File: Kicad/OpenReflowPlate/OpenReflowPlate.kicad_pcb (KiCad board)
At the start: 2 copper layers, 7 parts, among them U1 STM32L476RGTx

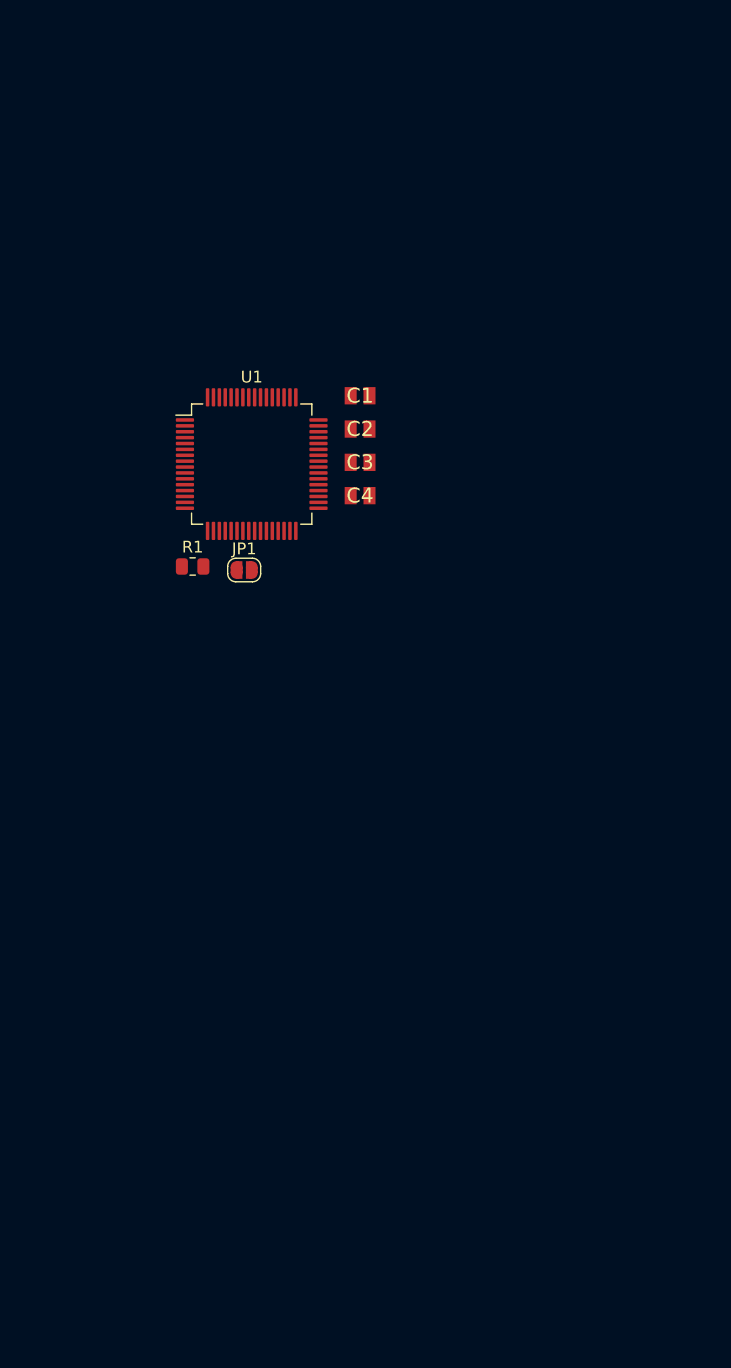
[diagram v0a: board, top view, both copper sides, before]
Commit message: last version
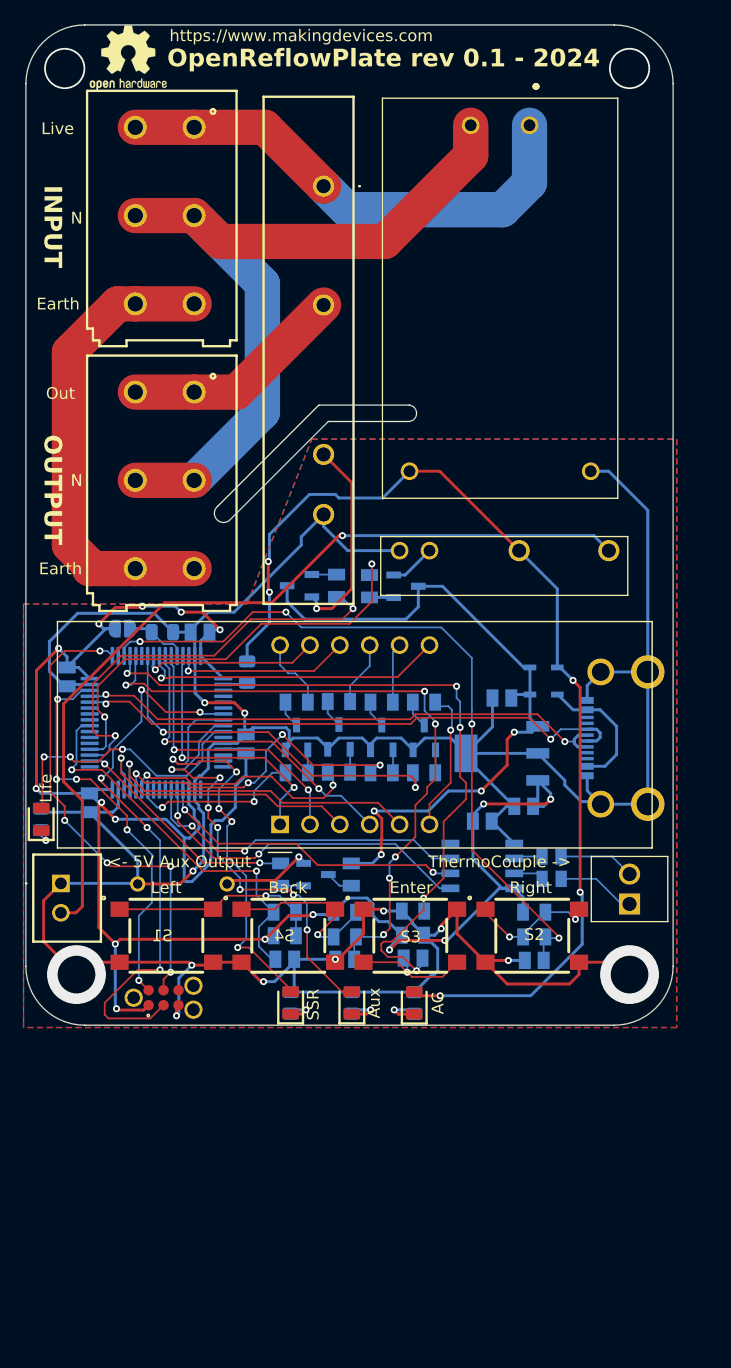
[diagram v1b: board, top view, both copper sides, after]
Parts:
- added AC/DC 3w: HLK-PM03, User_lib:HLKPM03, F.Cu at (129.5, 25.8)
- added Buzzer: TMB12A05, User_lib:TMB12A05, B.Cu at (103.8, 90.3)
- added C1: 100nF, User_lib:CAPC2012X140N, B.Cu at (125.5, 85.0)
- added C10: 22pF, User_lib:CAPC2012X140N, B.Cu at (113.8, 96.7)
- added C11: 22pF, User_lib:CAPC2012X140N, B.Cu at (119.6, 96.6)
- added C2: 100nF, User_lib:CAPC2012X140N, B.Cu at (127.2, 74.5)
- added C3: 100nF, User_lib:CAPC2012X140N, B.Cu at (129.0, 83.7)
- added C8: 22pF, User_lib:CAPC2012X140N, B.Cu at (129.9, 96.8)
- added C9: 22pF, User_lib:CAPC2012X140N, B.Cu at (108.7, 96.7)
- added D1: ZLLS410TA, User_lib:SOD2513X120N, B.Cu at (130.7, 74.2)
- added D2: ZLLS410TA, User_lib:SOD2513X120N, B.Cu at (130.7, 71.9)
- added IC1: MAX31855KASA+, User_lib:SOIC127P600X175-8N, B.Cu at (125.5, 88.8)
- added IC2: TC1108-3.3VDBTR, User_lib:SOT230P700X180-4N, B.Cu at (127.2, 79.2)
- added J1: TC connector, User_lib:282834-2_1, F.Cu at (138.0, 92.0)
- added J2: B2B-XH-A, User_lib:B2BXHA, F.Cu at (89.7, 90.2)
- added J3: Output_AC, User_lib:691411910003, F.Cu at (98.5, 56.0)
- added J4: Input_AC, User_lib:691411910003, F.Cu at (98.5, 33.5)
- added J5: Type - C, User_lib:2169900003, B.Cu at (138.4, 77.9)
- added K1: SSRC-240D5R, User_lib:SSRC240D5R, F.Cu at (112.0, 31.0)
- added K2: HF49FD_012-1H12F, User_lib:HF49FD0121H12F, F.Cu at (136.2, 62.0)
- added LED1: SML-H12V8TT86, User_lib:LEDC2012X90N, F.Cu at (119.7, 100.4)
- added LED2: SML-H12V8TT86, User_lib:LEDC2012X90N, F.Cu at (109.2, 100.4)
- added LED3: SML-H12V8TT86, User_lib:LEDC2012X90N, F.Cu at (114.4, 100.4)
- added LED4: SML-H12V8TT86, User_lib:LEDC2012X90N, F.Cu at (88.0, 84.8)
- added LFB1: Ferrite, User_lib:CAPC2012X90N, B.Cu at (131.4, 88.0)
- added LFB2: Ferrite, User_lib:CAPC2012X90N, B.Cu at (131.4, 89.9)
- added Q1: SMMBT5551LT1G, User_lib:SOT96P237X111-3N, B.Cu at (109.7, 77.8)
- added Q2: SMMBT5551LT1G, User_lib:SOT96P237X111-3N, B.Cu at (113.3, 77.8)
- added Q3: SMMBT5551LT1G, User_lib:SOT96P237X111-3N, B.Cu at (116.9, 77.8)
- added Q4: SMMBT5551LT1G, User_lib:SOT96P237X111-3N, B.Cu at (120.6, 77.8)
- added Q5: SMMBT5551LT1G, User_lib:SOT96P237X111-3N, B.Cu at (111.3, 89.5)
- added Q6: SMMBT5551LT1G, User_lib:SOT96P237X111-3N, B.Cu at (110.0, 65.0)
- added Q7: SMMBT5551LT1G, User_lib:SOT96P237X111-3N, B.Cu at (119.0, 65.0)
- added R1: 4k7, User_lib:RESC2012X65N, B.Cu at (109.7, 80.8)
- added R10: 100, User_lib:RESC2012X65N, B.Cu at (116.9, 74.8)
- added R11: 4k7, User_lib:RESC2012X65N, B.Cu at (120.5, 80.8)
- added R12: 100, User_lib:RESC2012X65N, B.Cu at (120.5, 74.8)
- added R13: 0, Resistor_SMD:R_0805_2012Metric, B.Cu at (105.5, 72.3)
- added R15: 10k, User_lib:RESC2012X75N, B.Cu at (129.9, 94.8)
- added R16: 10k, User_lib:RESC2012X75N, B.Cu at (108.7, 94.7)
- added R17: 10K, User_lib:RESC2012X65N, B.Cu at (108.7, 92.7)
- added R18: 10k, User_lib:RESC2012X65N, B.Cu at (129.9, 92.7)
- added R19: 4k7, User_lib:RESC2012X65N, B.Cu at (108.3, 89.5)
- added R2: 1k, Resistor_SMD:R_0805_2012Metric, B.Cu at (119.7, 100.4)
- added R20: 220, User_lib:RESC2012X65N, B.Cu at (114.3, 89.5)
- added R21: 10K, User_lib:RESC2012X75N, B.Cu at (119.6, 92.6)
- added R22: 10k, User_lib:RESC2012X75N, B.Cu at (113.8, 94.8)
- added R23: 4k7, User_lib:RESC2012X65N, B.Cu at (113.1, 65.0)
- added R24: 10k, User_lib:RESC2012X65N, B.Cu at (119.6, 94.7)
- added R25: 10k, User_lib:RESC2012X65N, B.Cu at (113.8, 92.7)
- added R26: 4k7, User_lib:RESC2012X65N, B.Cu at (115.9, 65.0)
- added R3: 100, User_lib:RESC2012X65N, B.Cu at (109.7, 74.8)
- added R4: 220, Resistor_SMD:R_0805_2012Metric, B.Cu at (109.2, 100.4)
- added R5: 4k7, User_lib:RESC2012X65N, B.Cu at (113.3, 80.8)
- added R6: 100, User_lib:RESC2012X65N, B.Cu at (113.3, 74.8)
- added R7: 220, Resistor_SMD:R_0805_2012Metric, B.Cu at (114.4, 100.4)
- added R8: 220, Resistor_SMD:R_0805_2012Metric, B.Cu at (88.0, 84.8)
- added R9: 4k7, User_lib:RESC2012X65N, B.Cu at (116.9, 80.8)
- added REF**: OSHW-Logo2_7.3x6mm_SilkScreen, Symbol:OSHW-Logo2_7.3x6mm_SilkScreen, F.Cu at (95.4, 20.1)
- added S1: Left Button, User_lib:430182070816, F.Cu at (98.6, 94.7)
- added S2: Right Button, User_lib:430182070816, F.Cu at (129.7, 94.7)
- added S3: Enter Button, User_lib:430182070816, F.Cu at (119.4, 94.7)
- added S4: Back Button, User_lib:430182070816, F.Cu at (109.0, 94.7)
- added SWD: TC2030-MCP-NL, User_lib:TC2030-MCP-NL, F.Cu at (98.4, 100.0)
- added U1: CC56-12EWA, Display_7Segment:CA56-12EWA, F.Cu at (108.3, 85.2)
- C4: renamed from C1; moved to B.Cu
- C5: renamed from C2; moved to B.Cu
- C6: renamed from C3; moved to B.Cu
- C7: renamed from C4; moved to B.Cu
- JP1: moved to B.Cu
- R14: renamed from R1; moved to B.Cu
- U2: renamed from U1; moved to B.Cu
- moved C7 34.8 mm to (92.1, 83.4), turned to 90 degrees
- moved C5 32.6 mm to (90.2, 72.7), turned to 90 degrees
- moved C4 31.1 mm to (105.4, 78.4), turned to -90 degrees
- moved U2 23.4 mm to (97.8, 76.6), turned to 180 degrees
- moved C6 19.8 mm to (101.5, 68.9)
- moved JP1 11.5 mm to (94.9, 68.6)
- moved R14 6.14 mm to (98.3, 68.9), turned to 180 degrees
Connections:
- U2 pad 10: unconnected-(U1-PC2-Pad10) -> LED_LIFE
- U2 pad 2: unconnected-(U1-PC13-Pad2) -> Net-(U2-PC13)
- U2 pad 20: unconnected-(U1-PA4-Pad20) -> SPI1_NSS
- U2 pad 21: unconnected-(U1-PA5-Pad21) -> SPI_CLK
- U2 pad 22: unconnected-(U1-PA6-Pad22) -> SPI_MISO
- U2 pad 26: unconnected-(U1-PB0-Pad26) -> C_1
- U2 pad 27: unconnected-(U1-PB1-Pad27) -> C_2
- U2 pad 28: unconnected-(U1-PB2-Pad28) -> C_3
- U2 pad 29: unconnected-(U1-PB10-Pad29) -> D_g
- U2 pad 30: unconnected-(U1-PB11-Pad30) -> D_dp
- U2 pad 34: unconnected-(U1-PB13-Pad34) -> C_buzzer
- U2 pad 35: unconnected-(U1-PB14-Pad35) -> C_out1
- U2 pad 36: unconnected-(U1-PB15-Pad36) -> C_out2
- U2 pad 40: unconnected-(U1-PC9-Pad40) -> BUT_LEFT
- U2 pad 51: unconnected-(U1-PC10-Pad51) -> BUT_RIGHT
- U2 pad 52: unconnected-(U1-PC11-Pad52) -> BUT_ENTER
- U2 pad 53: unconnected-(U1-PC12-Pad53) -> BUT_BACK
- U2 pad 55: unconnected-(U1-PB3-Pad55) -> C_4
- U2 pad 56: unconnected-(U1-PB4-Pad56) -> D_a
- U2 pad 57: unconnected-(U1-PB5-Pad57) -> D_b
- U2 pad 58: unconnected-(U1-PB6-Pad58) -> D_c
- U2 pad 59: unconnected-(U1-PB7-Pad59) -> D_d
- U2 pad 61: unconnected-(U1-PB8-Pad61) -> D_e
- U2 pad 62: unconnected-(U1-PB9-Pad62) -> D_f
- U2 pad 7: unconnected-(U1-NRST-Pad7) -> reset
- U2 pad 8: unconnected-(U1-PC0-Pad8) -> LED_OUT1
- U2 pad 9: unconnected-(U1-PC1-Pad9) -> LED_OUT2
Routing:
- net GND: track 0.00 -> 299.6 mm, vias 0 -> 12
- net +3V3: track 0.00 -> 171.4 mm, vias 0 -> 16
- net AC_Vdcin+: track 0.00 -> 90.2 mm, vias 0 -> 5
- net DC_Out2: track 0.00 -> 72.7 mm, vias 0 -> 1
- net AC_N: track 0.00 -> 67.3 mm
- net BUT_RIGHT: track 0.00 -> 63.2 mm, vias 0 -> 4
- net BUT_ENTER: track 0.00 -> 62.3 mm, vias 0 -> 5
- net +5V: track 0.00 -> 59.7 mm, vias 0 -> 4
- net BUT_BACK: track 0.00 -> 56.1 mm, vias 0 -> 6
- net reset: track 0.00 -> 47.6 mm, vias 0 -> 5
- net USB_D-: track 0.00 -> 47.4 mm, vias 0 -> 2
- net USB_D+: track 0.00 -> 46.1 mm, vias 0 -> 2
- net AC_L: track 0.00 -> 42.2 mm
- net SWCLK: track 0.00 -> 41.0 mm, vias 0 -> 5
- net AC_ground: track 0.00 -> 40.3 mm
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- added copper zone on B.Cu, net GND
- added copper zone on F.Cu, net GND
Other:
- board outline added: 55 x 85 mm
- board text added: "+"
- board text added: "-"
- board text added: "5V"
- board text added: "<- 5V Aux Output"
- board text added: "AC"
- board text added: "AC/DC 3W"
- board text added: "Aux"
- board text added: "Back"
- board text added: "Danger - Main Voltage"
- board text added: "Earth"
- board text added: "Enter"
- board text added: "GND"
- board text added: "INPUT"
- board text added: "LDO"
- board text added: "Left"
- board text added: "Life"
- board text added: "Live"
- board text added: "Live - in"
- board text added: "Live - out"
- board text added: "MAX"
- board text added: "N"
- board text added: "Neutral"
- board text added: "OUTPUT"
- board text added: "OpenReflowPlate rev 0.1 - 2024"
- board text added: "Out"
- board text added: "Right"
- board text added: "SSR"
- board text added: "STM32L476RG"
- board text added: "SWD"
- board text added: "ThermoCouple ->"
- board text added: "Type-C"
- board text added: "https://www.makingdevices.com"

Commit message: V1 HW
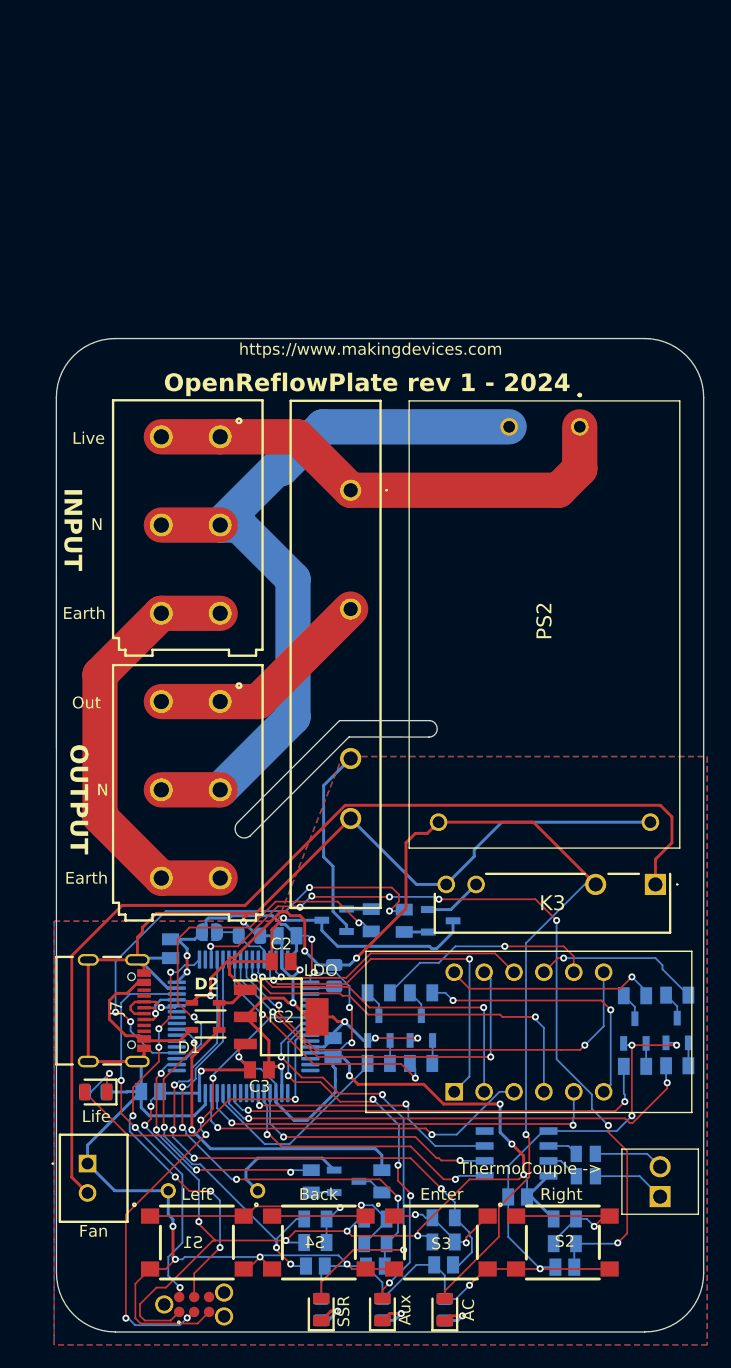
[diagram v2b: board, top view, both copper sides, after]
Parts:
- removed AC/DC 3w: HLK-PM03, User_lib:HLKPM03
- removed J5: Type - C, User_lib:2169900003
- removed K2: HF49FD_012-1H12F, User_lib:HF49FD0121H12F
- removed REF**: OSHW-Logo2_7.3x6mm_SilkScreen, Symbol:OSHW-Logo2_7.3x6mm_SilkScreen
- added J7: 629722000214, usb-c:629722000214, F.Cu at (92.0, 101.1)
- added K3: HF49FD_012-1H11F, User_3:HF49FD0121H11F, F.Cu at (140.2, 90.3)
- added PS2: HLK-5M05, User_3:HLK5M05, F.Cu at (133.8, 51.5)
- C2, C3, D1, D2, IC2: moved to F.Cu
- moved D1 40.5 mm to (102.0, 102.7), turned to 180 degrees
- moved D2 40.5 mm to (102.0, 100.4), turned to 180 degrees
- moved R1 38.1 mm to (138.5, 105.8)
- moved R3 38.1 mm to (138.5, 99.8)
- moved Q1 38.1 mm to (138.5, 102.8)
- moved Q2 38.1 mm to (142.1, 102.8)
- moved R5 38.1 mm to (142.1, 105.8)
- moved R6 38.1 mm to (142.1, 99.8)
- moved C1 32.1 mm to (128.5, 116.9), turned to 180 degrees
- moved C3 31.7 mm to (106.5, 106.1), turned to 0 degrees
- moved C2 29.2 mm to (108.4, 96.9), turned to 0 degrees
- moved IC2 29.2 mm to (108.4, 101.6), turned to 0 degrees
- moved Q6 28.6 mm to (112.9, 93.4)
- moved Q7 28.6 mm to (122.0, 93.4)
- moved R23 28.6 mm to (116.0, 93.4)
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- renumbered SWD to J6, Buzzer to LS1
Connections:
- C11 pad 2: Net-(C11-Pad2) -> GND
- R21 pad 2: GND -> Net-(R21-Pad2)
- R24 pad 1: GND -> Net-(R21-Pad2)
- S3 pad 1: GND -> Net-(R21-Pad2)
- S3 pad 2: Net-(C11-Pad2) -> GND
- S3 pad 3: GND -> Net-(R21-Pad2)
- S3 pad 4: Net-(C11-Pad2) -> GND
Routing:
- net USB_D-: track 47.4 -> 5.93 mm, vias 2 -> 1
- net USB_D+: track 46.1 -> 5.45 mm, vias 2 -> 1
- net GND: track 299.6 -> 265.9 mm, vias 12 -> 16
- net C_1: track 14.5 -> 37.6 mm
- net C_2: track 20.5 -> 42.0 mm
- net D_a: track 15.4 -> 33.1 mm, vias 1 -> 2
- net D_b: track 26.2 -> 40.2 mm, vias 1 -> 2
- net CC_3: track 5.09 -> 19.0 mm, vias 0 -> 1
- net BUT_BACK: track 56.1 -> 43.3 mm, vias 6 -> 4
- net CC_1: track 6.18 -> 18.3 mm, vias 0 -> 1
- net BUT_ENTER: track 62.3 -> 50.3 mm, vias 5 -> 4
- net +3V3: track 171.4 -> 159.6 mm, vias 16 -> 18
- net DC_Out2: track 72.7 -> 83.7 mm, vias 1 -> 0
- net CC_4: track 12.2 -> 23.0 mm, vias 1 -> 2
- net Net-(C11-Pad2): track 10.3 -> 0.00 mm, vias 1 -> 0
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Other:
- board size 55 x 85 mm -> 55 x 84.4 mm
- board text added: "Fan"
- board text added: "OpenReflowPlate rev 1 - 2024"
- board text removed: "<- 5V Aux Output"
- board text removed: "OpenReflowPlate rev 0.1 - 2024"
